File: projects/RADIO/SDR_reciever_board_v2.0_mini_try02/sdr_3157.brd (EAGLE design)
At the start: 60 x 75 mm, 56 parts, among them IC1 LM1117-33, U1 NE5532D, U2 SN74LVC1G3157DBVR, U3 SN74LVC1G3157DBVR

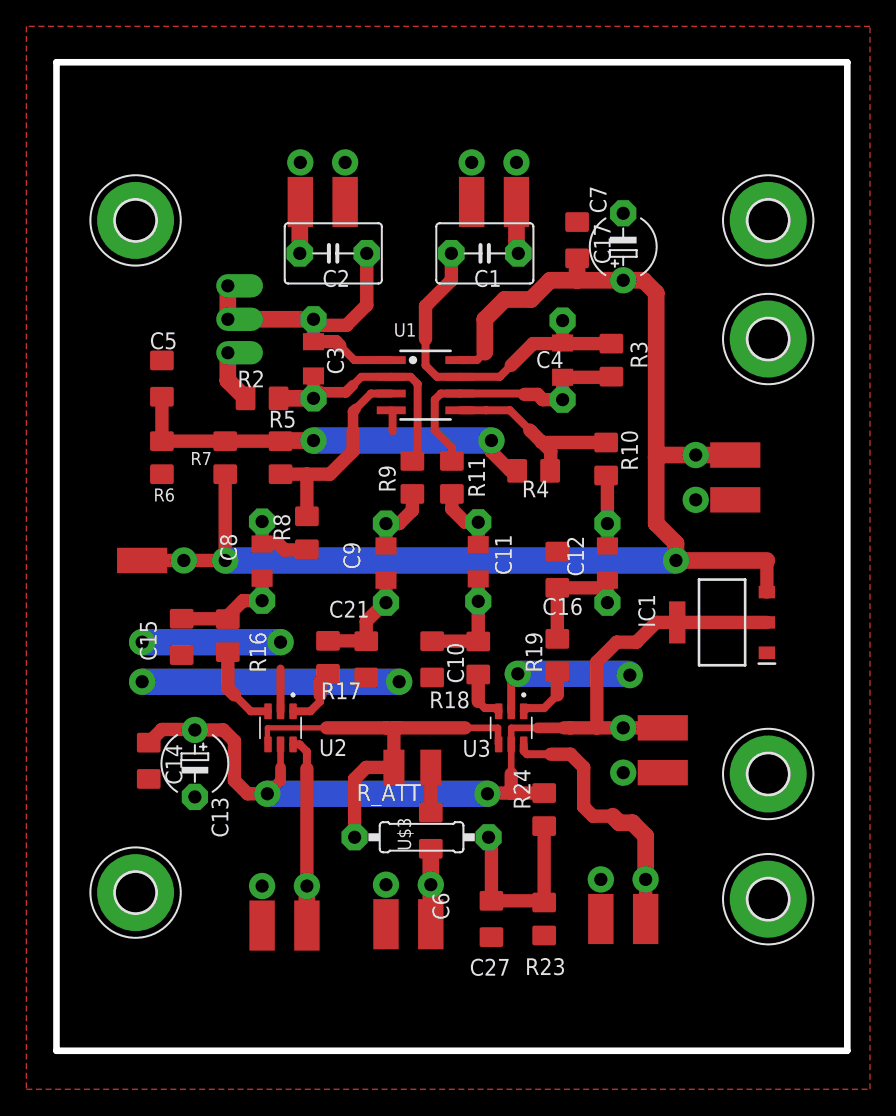
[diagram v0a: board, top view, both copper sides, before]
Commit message: update
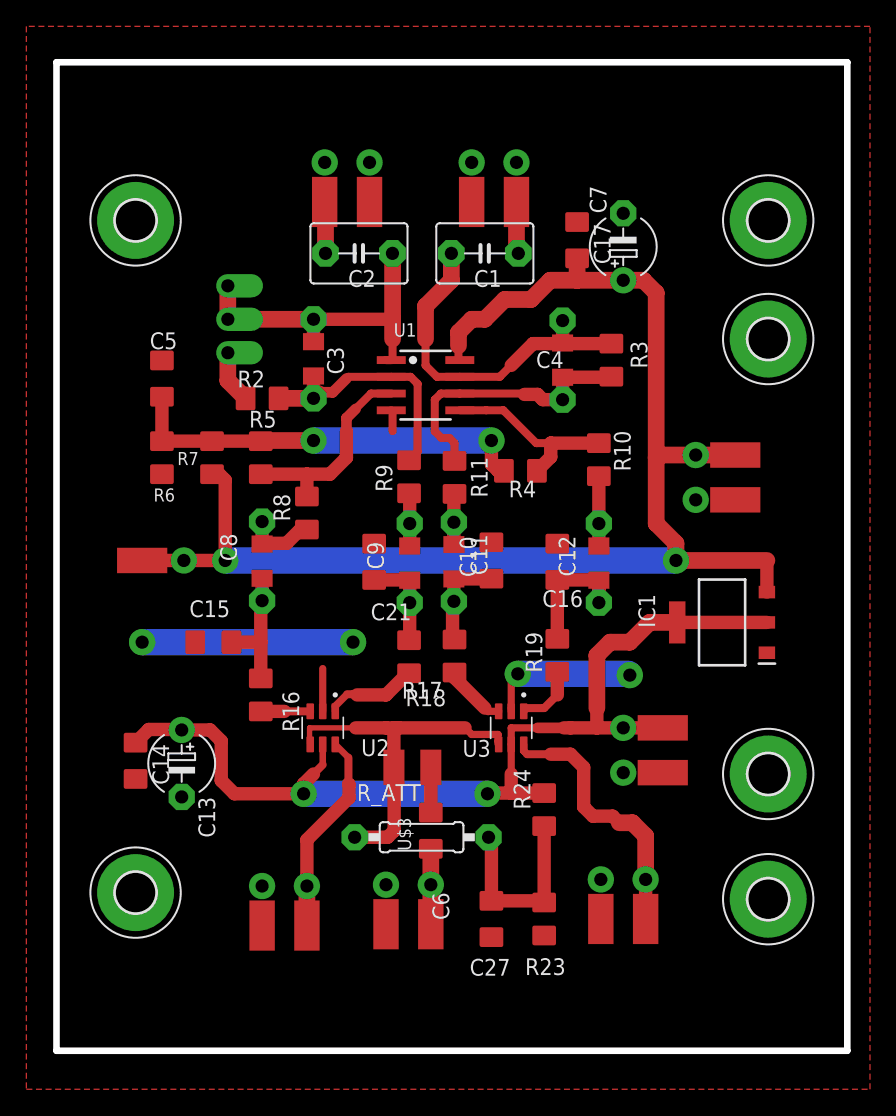
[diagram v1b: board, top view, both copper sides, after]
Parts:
- moved C10 8.75 mm to (33.0, 37.2), turned to 90 degrees
- moved C21 7.42 mm to (24.1, 37.1), turned to 270 degrees
- moved R17 6.15 mm to (26.8, 29.9)
- moved R16 5.15 mm to (15.5, 27.0)
- moved U2 3.20 mm to (20.2, 24.5)
- moved C15 2.43 mm to (11.9, 31.0), turned to 180 degrees
- moved C2 1.95 mm to (22.9, 60.5)
- moved C11 1.85 mm to (30.1, 37.1)
- moved Q 1.85 mm to (22.1, 64.4)
- moved R18 1.81 mm to (30.2, 29.9)
- moved C9 1.80 mm to (26.8, 37.0)
- moved R5 1.50 mm to (15.5, 45.0)
- moved R8 1.50 mm to (19.0, 40.8)
- moved C13 1.00 mm to (9.50, 21.8)
- moved C14 1.00 mm to (6.00, 22.0)
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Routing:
- net GND: track 46.5 -> 32.5 mm, vias 6 -> 4
- net ANTENNA: track 30.8 -> 27.6 mm
- net N$3: track 6.52 -> 3.75 mm
- net N$4: track 4.70 -> 7.18 mm
- net VCC: track 74.0 -> 75.5 mm
- net N$14: track 5.26 -> 3.87 mm
- net N$8: track 8.53 -> 9.92 mm
- net N$13: track 5.36 -> 4.02 mm
- net N$9: track 8.20 -> 7.28 mm
- net N$5: track 4.02 -> 4.80 mm
- net COS_IN: track 14.8 -> 15.5 mm
- net N$10: track 8.26 -> 7.56 mm
- net N$18: track 14.7 -> 14.1 mm
- net N$11: track 10.5 -> 11.0 mm
